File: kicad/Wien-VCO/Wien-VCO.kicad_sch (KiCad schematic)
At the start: 12 parts, among them U1 TL081

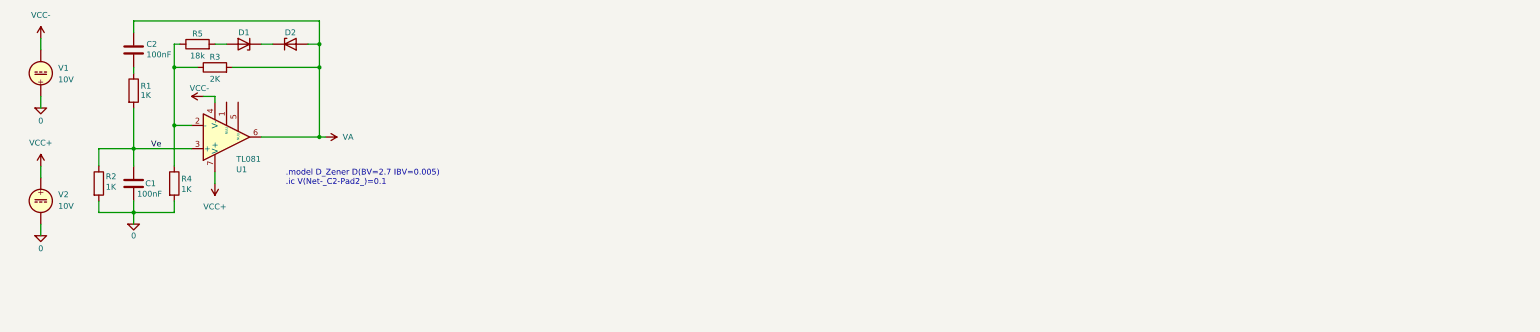
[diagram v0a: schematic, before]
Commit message: Wien-Brücken-Schwinger mit JFET zur Amplitudenstabilisierung
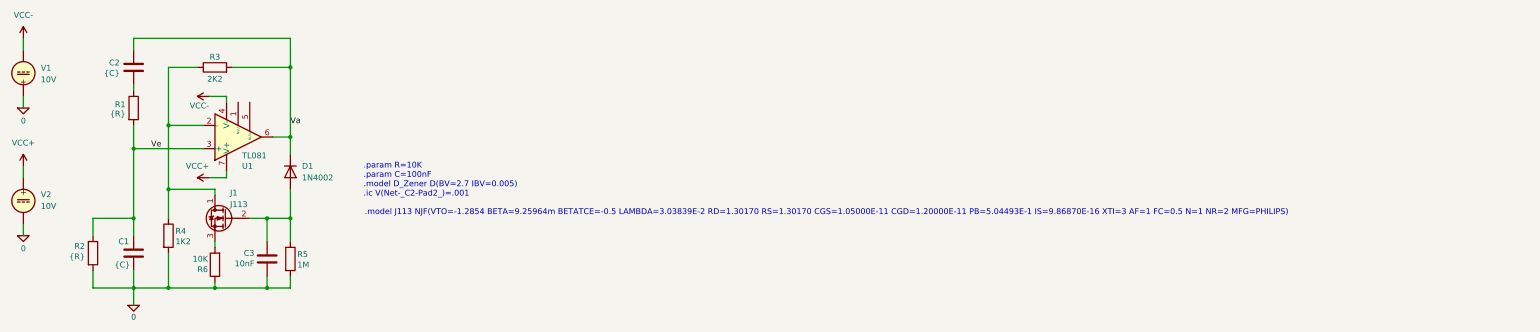
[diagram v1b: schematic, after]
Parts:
- removed D1, D2: D_Zener, symbol Device:D_Zener
- added C3: 10nF, symbol Device:C
- added D1: 1N4002, Diode_THT:D_DO-35_SOD27_P7.62mm_Horizontal, symbol Diode:1N4148
- added J1: J113, Package_TO_SOT_THT:TO-92_Inline, symbol Transistor_FET:BS170
- added R6: 10K, symbol Device:R
- C1, C2: value 100nF -> {C}
- R1, R2: value 1K -> {R}
- R3: value 2K -> 2K2
- R4: value 1K -> 1K2
- R5: value 18k -> 1M
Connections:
- net 0: now also R5.2, C3.1, R6.1
- net at R3.1, R4.1, U1.2 (-): now also J1.1 (D); no longer R5.1
- net VA renamed Va
- net Va: now also D1.1 (K)
- new net: C3.2, D1.2 (A), J1.2 (G), R5.1
- new net: J1.3 (S), R6.2
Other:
- note added: ".model J113 NJF(VTO=-1.2854 BETA=9.25964m BETATCE=-0.5 LAMBDA=3.03839E-2 RD=1.30170 RS=1.30170 CGS=1.05000E-11 CGD=1.20000E-11 PB=5.04493E-1 IS=9.86870E-16 XTI=3 AF=1 FC=0.5 N=1 NR=2 MFG=PHILIPS)"
- note added: ".param R=10K .param C=100nF .model D_Zener D(BV=2.7 IBV=0.005) .ic V(Net-_C2-Pad2_)=.001"
- note removed: ".model D_Zener D(BV=2.7 IBV=0.005) .ic V(Net-_C2-Pad2_)=0.1"
- moved on the sheet: C1, C2, R1, R2, R4, U1, V1, V2
